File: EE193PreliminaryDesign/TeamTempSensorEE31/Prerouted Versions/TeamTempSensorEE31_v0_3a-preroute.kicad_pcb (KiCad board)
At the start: 2 copper layers, 27.4 x 62.2 mm, 39 parts, among them J1 USB_B_Micro, J2 Battery_Connector, Q1 BS170F, Q2 BC818, Q3 BC818, Q4 NTA4151PT1G, SW1 SW_DIP_x01, U1 CP2102N-A02-GQFN28, U2 MCP9808_MSOP, U3 LD1117S33TR_SOT223, U4 ESP32-C3-WROOM-02

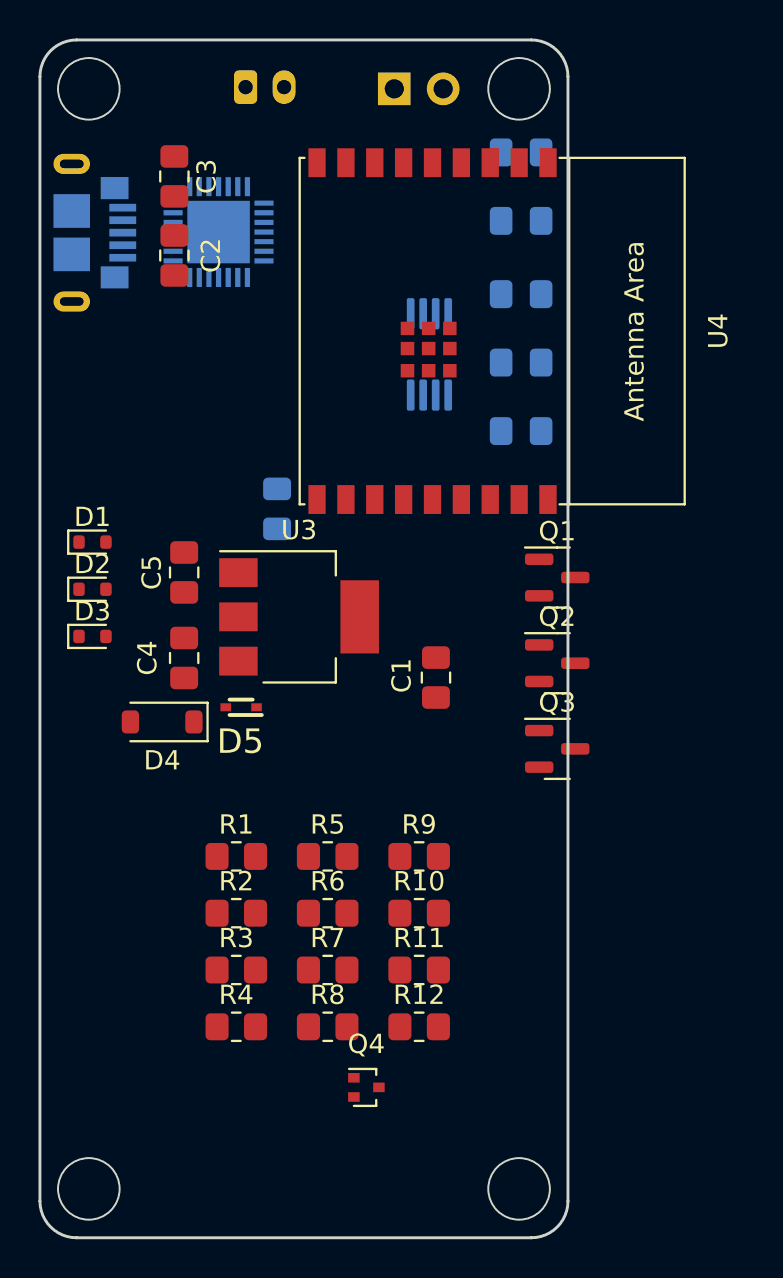
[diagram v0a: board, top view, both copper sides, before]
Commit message: v0.4 complete layout
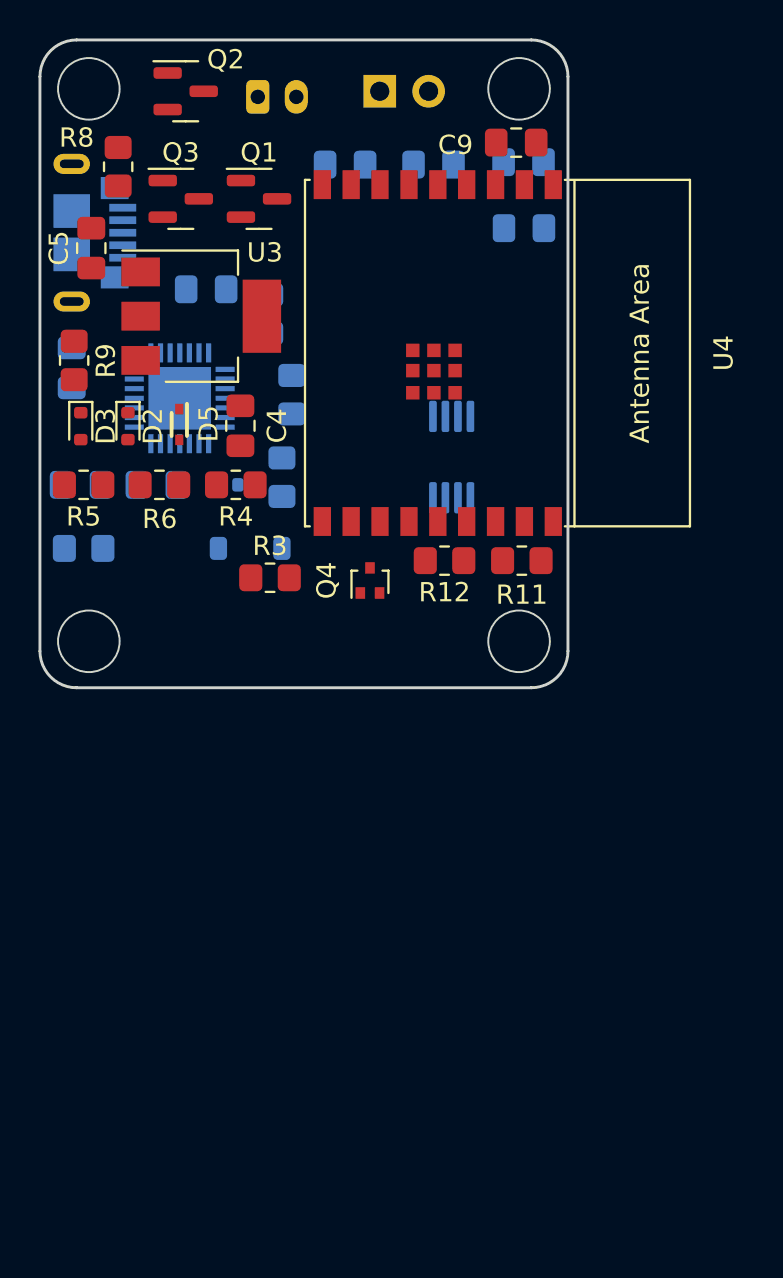
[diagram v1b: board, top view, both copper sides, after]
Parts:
- C1, C2, C3, D1, D4, R1, R10, R2, R7: moved to B.Cu
- C9: moved to F.Cu
- moved R8 46.0 mm to (170.3, 63.7), turned to -90 degrees
- moved Q2 35.4 mm to (173.8, 59.8)
- moved Q3 34.6 mm to (173.6, 65.4)
- moved R7 34.2 mm to (178.2, 71.4), turned to 90 degrees
- moved R9 31.4 mm to (168.0, 73.8), turned to 90 degrees
- moved R4 28.2 mm to (176.4, 80.3), turned to 180 degrees
- moved R2 27.1 mm to (179.3, 75.6), turned to -90 degrees
- moved Q4 26.3 mm to (183.4, 85.2), turned to 90 degrees
- moved R10 25.7 mm to (168.5, 83.6)
- moved Q1 25.0 mm to (177.6, 65.4)
- moved R12 24.3 mm to (187.3, 84.2), turned to 180 degrees
- moved R6 23.9 mm to (172.4, 80.3)
- moved C1 23.4 mm to (174.9, 70.1), turned to 180 degrees
- moved R5 23.1 mm to (168.5, 80.3), turned to 180 degrees
- moved R11 21.9 mm to (191.3, 84.2)
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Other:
- board size 27.4 x 62.2 mm -> 27.4 x 33.7 mm
